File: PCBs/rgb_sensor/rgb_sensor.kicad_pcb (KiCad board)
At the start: 2 copper layers, 25.3 x 6.1 mm, 10 parts, among them J1 Conn_01x05, Q1 AO3401A, U1 VEML3328

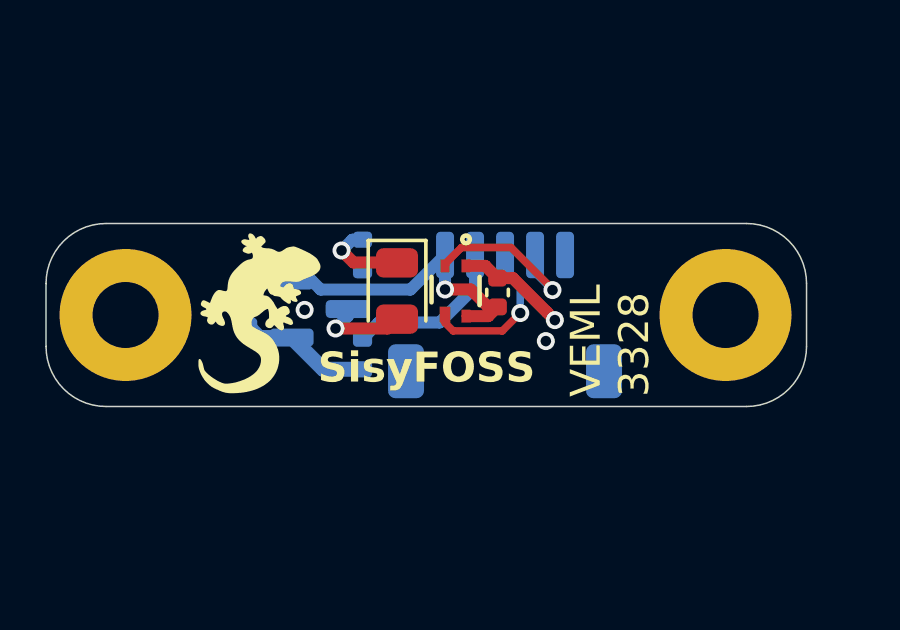
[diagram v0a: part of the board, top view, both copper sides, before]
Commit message: Initial changes for Gamma RGB sensor board
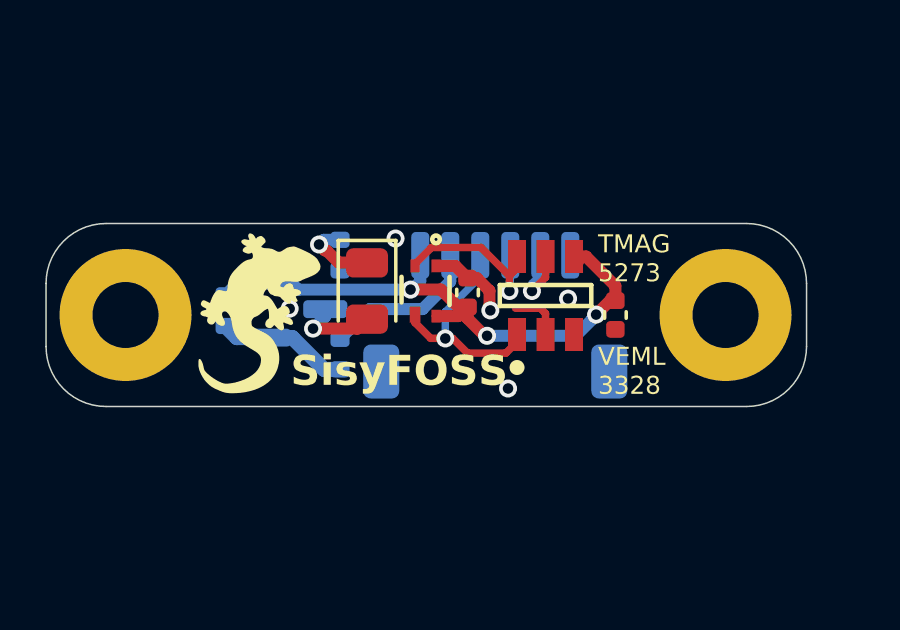
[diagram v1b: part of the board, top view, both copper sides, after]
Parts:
- added C2: 100n, Capacitor_SMD:C_0402_1005Metric, F.Cu at (151.8, 104.8)
- added U2: TMAG5273A1QDBVR, rgb_sensor:DBV0006A-MFG, F.Cu at (149.5, 104.2)
- J1: value Conn_01x05 -> Conn_01x06_MountingPin; footprint Connector_JST:JST_SH_SM05B-SRSS-TB_1x05-1MP_P1.00mm_Horizontal -> Connector_JST:JST_SH_SM06B-SRSS-TB_1x06-1MP_P1.00mm_Horizontal
- moved C1 1.00 mm to (146.9, 104.0)
- moved D1 1.00 mm to (143.6, 104.0)
- moved U1 1.00 mm to (145.5, 104.0)
- moved Q1 0.75 mm to (141.2, 104.6)
- moved R1 0.75 mm to (138.8, 104.7)
- moved R2 0.75 mm to (142.7, 106.1)
- moved R3 0.75 mm to (142.7, 102.8)
- moved J1 0.33 mm to (147.8, 104.8)
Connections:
- J1 pad 2: /SDA -> /INT_HALL
- J1 pad 3: /SCL -> /SDA
- J1 pad 4: /AUX_LED -> /SCL
- J1 pad 5: +3V3 -> /AUX_LED
- J1 pad MP: (no net) -> GND
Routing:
- net +3V3: track 11.7 -> 19.4 mm, vias 1 -> 3
- net /INT_HALL: track 0.00 -> 2.64 mm, vias 0 -> 1
- net /SCL: track 5.28 -> 7.75 mm
- net GND: track 3.65 -> 4.36 mm, vias 3 -> 5
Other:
- board text added: "TMAG 5273"
